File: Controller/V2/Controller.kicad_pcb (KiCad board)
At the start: 2 copper layers, 95.9 x 75.1 mm, 25 parts, among them J1 CONN_02X08, J10 CONN_01X02, J2 CONN_01X04, J3 CONN_01X02, J4 CONN_01X02, J5 CONN_01X02, J6 CONN_01X02, J7 CONN_01X02, J8 CONN_01X03, J9 CONN_01X02, Q1 BS107, U1 ARDUINO_NANO, U2 7805, U3 MCP4728, U4 AD9850_DDS_Module, U5 RELAY-G5V-1

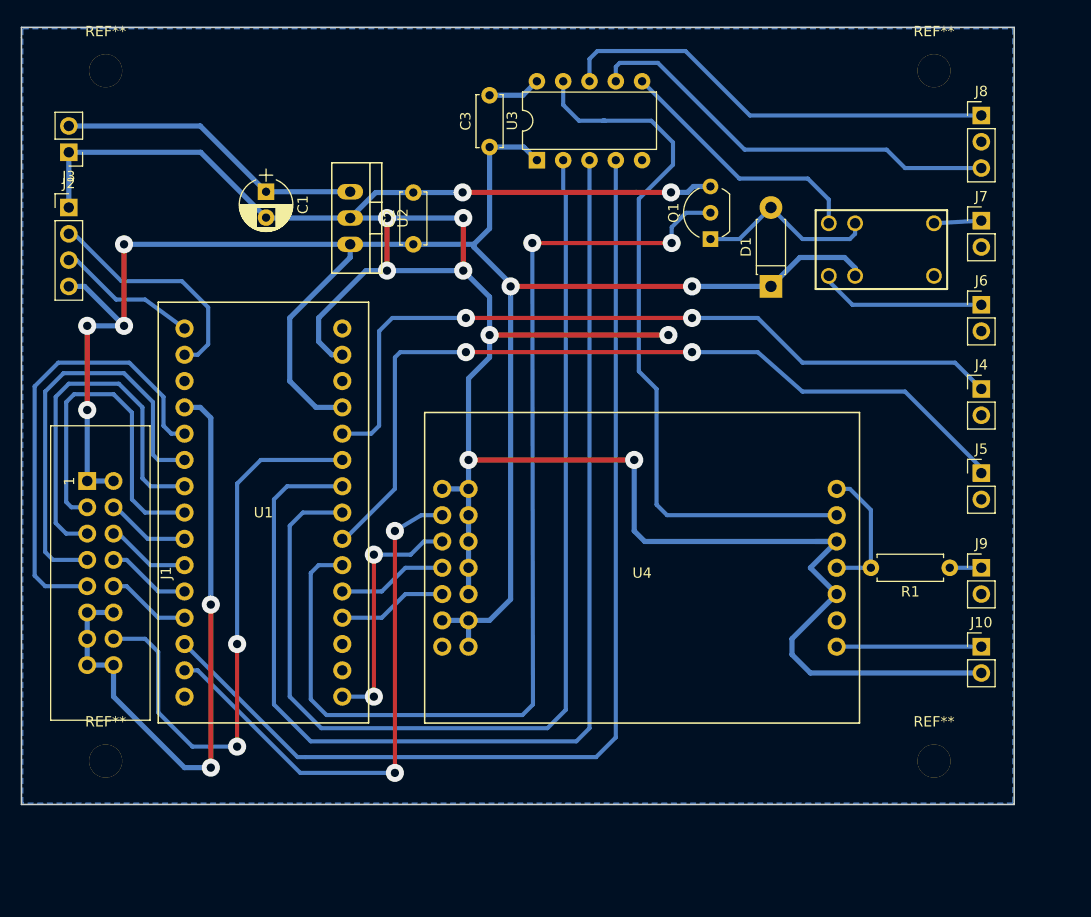
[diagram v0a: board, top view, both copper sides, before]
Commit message: Started to refactor code to use bettwe widget event handling Created UILib for use in future projects
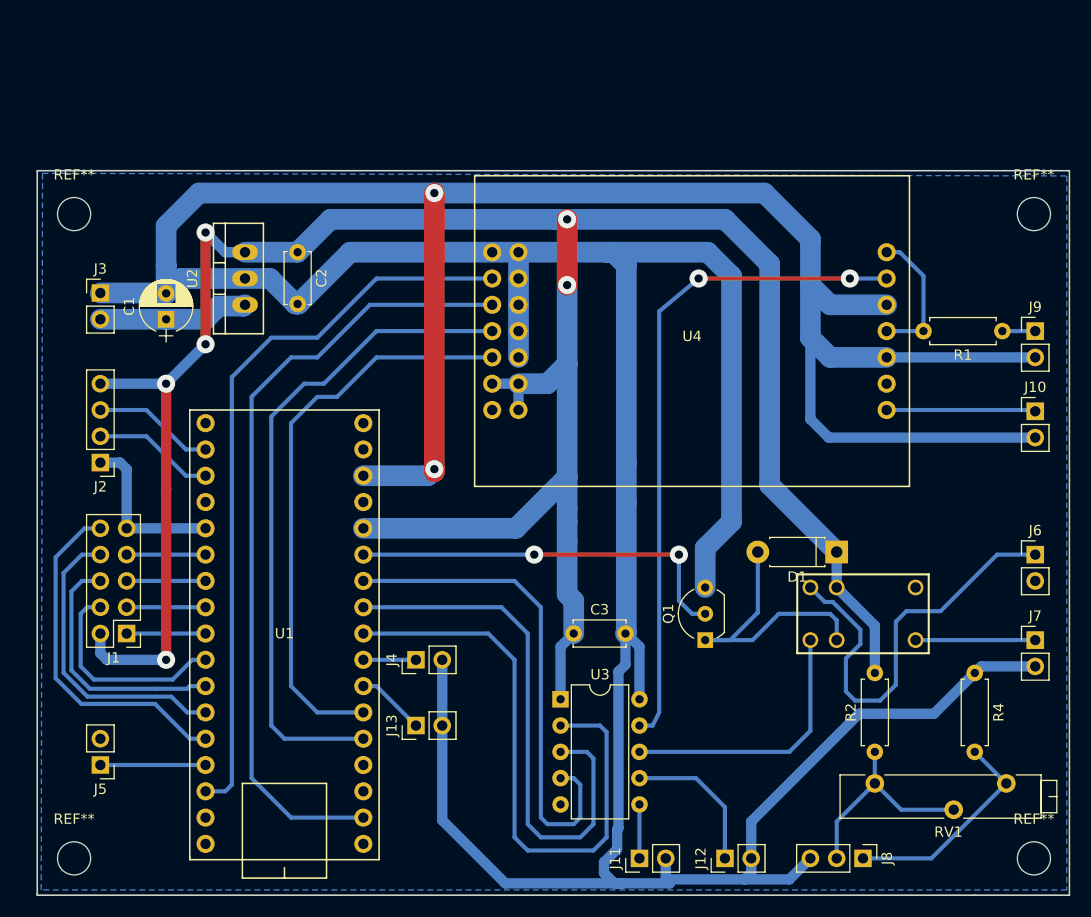
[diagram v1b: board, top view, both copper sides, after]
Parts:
- removed the REF** at (143.5, 106.9)
- removed the REF** at (63.5, 106.9)
- removed the REF** at (63.5, 173.6)
- removed the REF** at (143.5, 173.6)
- added J11: CONN_01X02, Pin_Headers:Pin_Header_Straight_1x02_Pitch2.54mm, F.Cu at (115.1, 183.0)
- added J12: CONN_01X02, Pin_Headers:Pin_Header_Straight_1x02_Pitch2.54mm, F.Cu at (123.3, 183.0)
- added J13: CONN_01X02, Pin_Headers:Pin_Header_Straight_1x02_Pitch2.54mm, F.Cu at (93.5, 170.2)
- added R2: R, Resistors_ThroughHole:R_Axial_DIN0207_L6.3mm_D2.5mm_P7.62mm_Horizontal, F.Cu at (137.8, 172.7)
- added R4: R, Resistors_ThroughHole:R_Axial_DIN0207_L6.3mm_D2.5mm_P7.62mm_Horizontal, F.Cu at (147.4, 165.1)
- added REF**: MountingHole_3.2mm_M3_DIN965, Mounting_Holes:MountingHole_3.2mm_M3_DIN965, F.Cu at (60.5, 120.8)
- added REF**: MountingHole_3.2mm_M3_DIN965, Mounting_Holes:MountingHole_3.2mm_M3_DIN965, F.Cu at (153.2, 120.8)
- added REF**: MountingHole_3.2mm_M3_DIN965, Mounting_Holes:MountingHole_3.2mm_M3_DIN965, F.Cu at (153.2, 183.0)
- added REF**: MountingHole_3.2mm_M3_DIN965, Mounting_Holes:MountingHole_3.2mm_M3_DIN965, F.Cu at (60.5, 183.0)
- added RV1: POT_TRIM, Potentiometers:Potentiometer_Trimmer_Bourns_3005, F.Cu at (137.8, 175.8)
- J1: value CONN_02X08 -> CONN_02X05; footprint Connect:IDC_Header_Straight_16pins -> Pin_Headers:Pin_Header_Straight_2x05_Pitch2.54mm
- moved J5 89.6 mm to (63.0, 174.0), turned to 180 degrees
- moved J8 72.7 mm to (136.7, 183.0), turned to 270 degrees
- moved J4 60.6 mm to (93.5, 163.8), turned to 90 degrees
- moved U3 52.1 mm to (107.4, 167.6), turned to 0 degrees
- moved C3 47.7 mm to (108.7, 161.3), turned to 0 degrees
- moved J7 40.8 mm to (153.3, 161.9)
- moved Q1 38.7 mm to (121.4, 161.9)
- moved U5 35.2 mm to (136.7, 159.4)
- moved D1 26.4 mm to (134.1, 153.4), turned to 180 degrees
- moved J2 24.8 mm to (63.0, 144.8), turned to 180 degrees
- moved J6 24.7 mm to (153.3, 153.7)
- moved J9 23.4 mm to (153.3, 132.1)
- moved R1 23.4 mm to (150.1, 132.1)
- moved U4 23.4 mm to (120.1, 132.1)
- moved J10 23.3 mm to (153.3, 139.8)
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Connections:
- J1 pad 1: +5V -> IO5
- J1 pad 3: IO5 -> IO4
- J1 pad 5: IO4 -> IO3
- J1 pad 7: IO3 -> IO2
- J1 pad 9: IO2 -> GND
- J8 pad 1: VO_REF1 -> VO_REF0
- J8 pad 2: GND -> VO_REF1
- J8 pad 3: VO_REF0 -> GND
- U1 pad 13: SEL_DAC_N -> VO_RANGE
- U1 pad 19: RST_DDS_N -> WR_DDS
- U1 pad 20: SEL_DDS_N -> RST_DDS
- U1 pad 21: VO_MOD_SEL -> AIN6
- U1 pad 22: VO_RANGE -> VI_PEAK
- U1 pad 25: AIN6 -> SEL_DAC_N
- U1 pad 26: VI_PEAK -> VO_MOD_SEL
- U3 pad 6: VO_AMP -> VO_OFFSET
- U3 pad 7: VO_REF0 -> VO_SWEEP
- U3 pad 8: VO_REF1 -> VO_AMP
- U4 pad 4: SEL_DDS_N -> WR_DDS
- U4 pad 5: RST_DDS_N -> RST_DDS
- U5 pad 1: Net-(J6-Pad1) -> VO_AMP
- U5 pad 10: VO_AMP -> Net-(J6-Pad1)
- U5 pad 2: +5V -> Net-(D1-Pad2)
- U5 pad 5: Net-(U5-Pad5) -> Net-(J7-Pad1)
- U5 pad 6: Net-(J7-Pad1) -> Net-(U5-Pad6)
- U5 pad 9: Net-(D1-Pad2) -> +5V
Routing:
- net GND: track 312.5 -> 467.8 mm, vias 12 -> 2
- net VO_RANGE: track 81.6 -> 10.2 mm, vias 2 -> 0
- net VI_PEAK: track 74.8 -> 5.08 mm, vias 2 -> 0
- net WR_DDS: track 0.00 -> 64.0 mm
- net VO_MOD_SEL: track 102.0 -> 38.0 mm
- net SDA: track 114.3 -> 52.5 mm
- net RST_DDS: track 0.00 -> 55.5 mm
- net SEL_DAC_N: track 102.7 -> 48.2 mm
- net SCK: track 23.9 -> 76.1 mm, vias 2 -> 0
- net +5V: track 188.7 -> 239.3 mm
- net AIN6: track 56.7 -> 6.66 mm, vias 2 -> 0
- net SCL: track 104.0 -> 57.6 mm
- net IO2: track 43.7 -> 7.62 mm
- net IO3: track 40.5 -> 7.62 mm
- net IO4: track 36.8 -> 7.62 mm
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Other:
- board size 95.9 x 75.1 mm -> 99.7 x 70 mm
- net class Power: trace_width 0.5 -> 1
